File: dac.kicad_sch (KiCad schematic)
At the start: 34 parts, among them U2 DAC61416RHAT

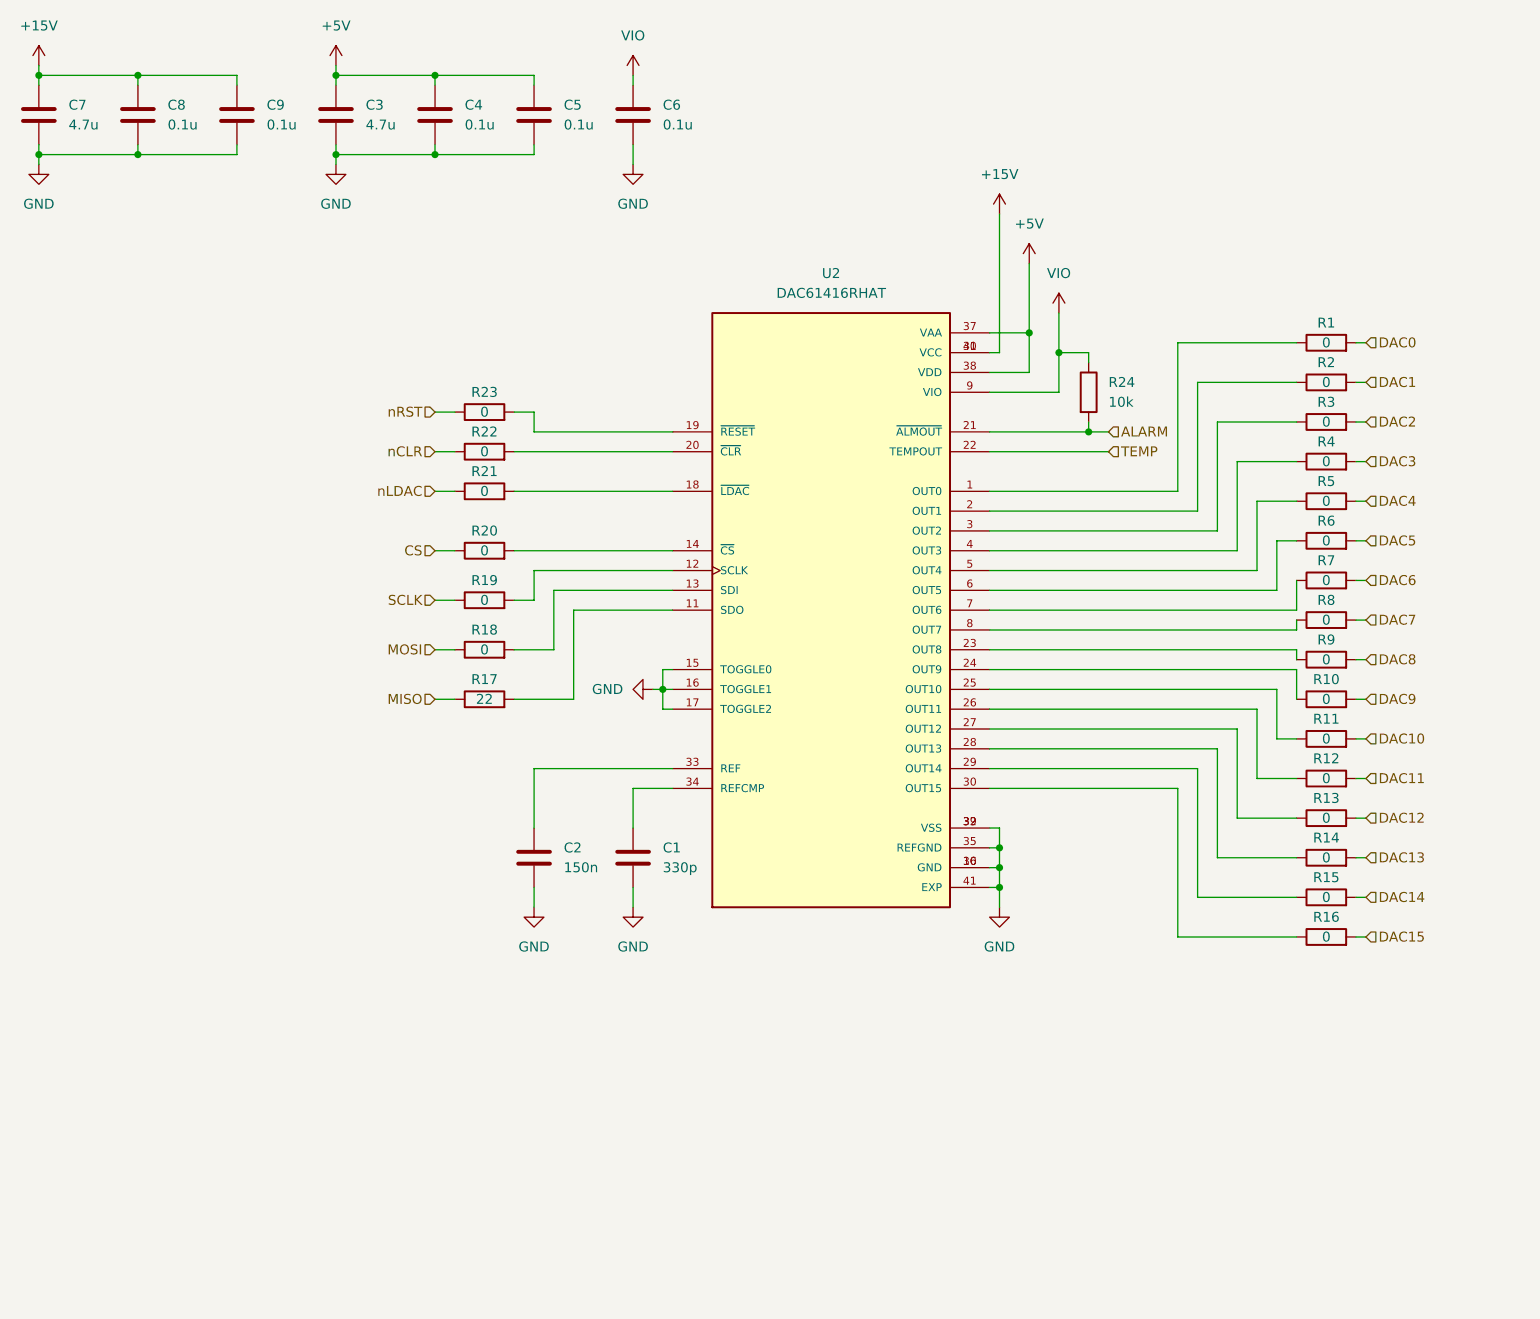
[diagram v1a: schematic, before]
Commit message: sch_0v1 ready for review
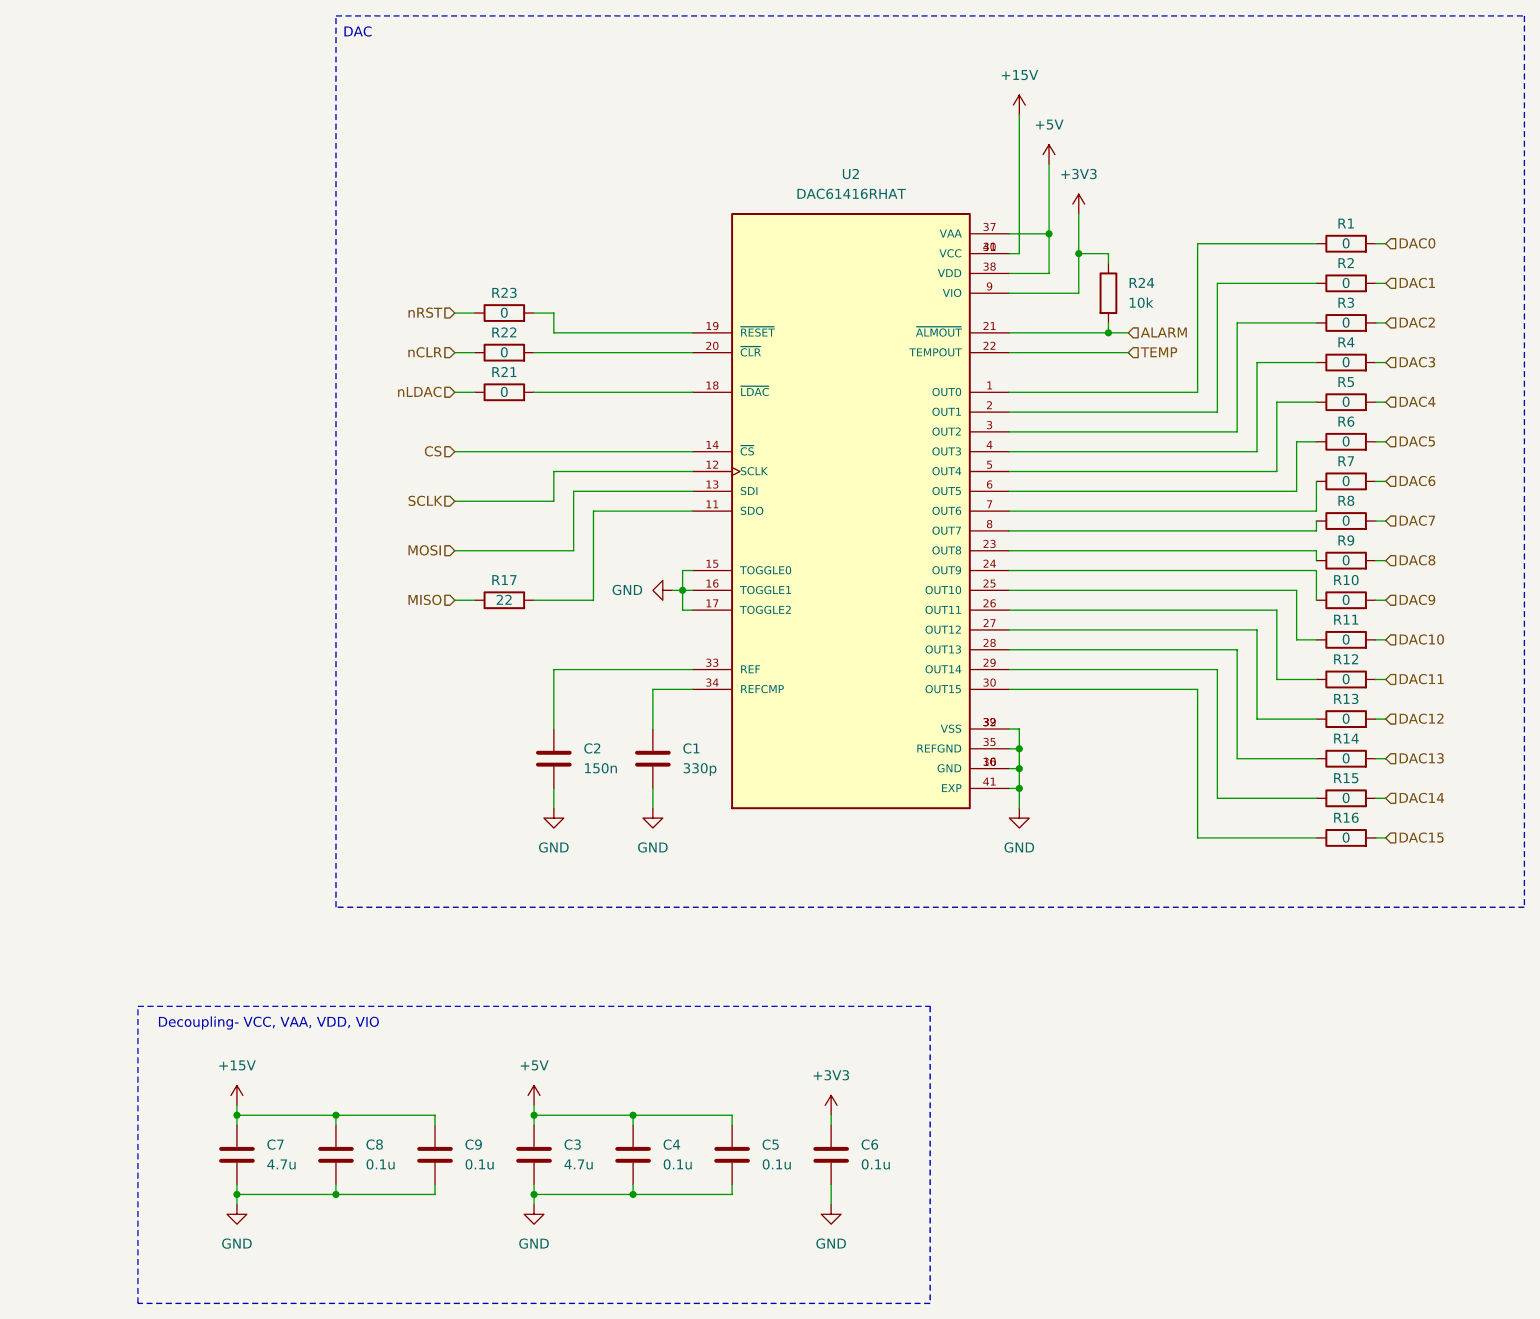
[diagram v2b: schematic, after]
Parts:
- removed R18, R19, R20: 0, symbol Device:R
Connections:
- net CS: now also U2.14 (~{CS})
- net MOSI: now also U2.13 (SDI)
- net SCLK: now also U2.12 (SCLK)
- net VIO renamed +3V3
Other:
- note added: "DAC"
- note added: "Decoupling- VCC, VAA, VDD, VIO"
- moved on the sheet: C1, C2, C3, C4, C5, C6, C7, C8, C9, R1, R10, R11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
